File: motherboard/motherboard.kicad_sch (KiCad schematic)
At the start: 37 parts, among them J1 Conn_01x20_Pin, J3 Conn_01x20_Pin, J4 USB2.0_16P, U1 74LS573, U3 74HC132, U4 74HC245, U5 74HC245, U6 HM62256BLP, U7 R6507, U8 NE555P, U9 74HC132

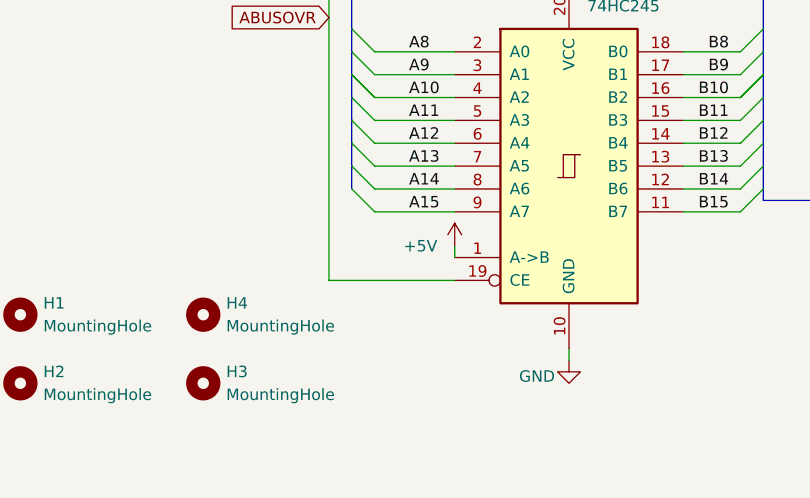
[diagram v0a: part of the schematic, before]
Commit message: Motherboard finished
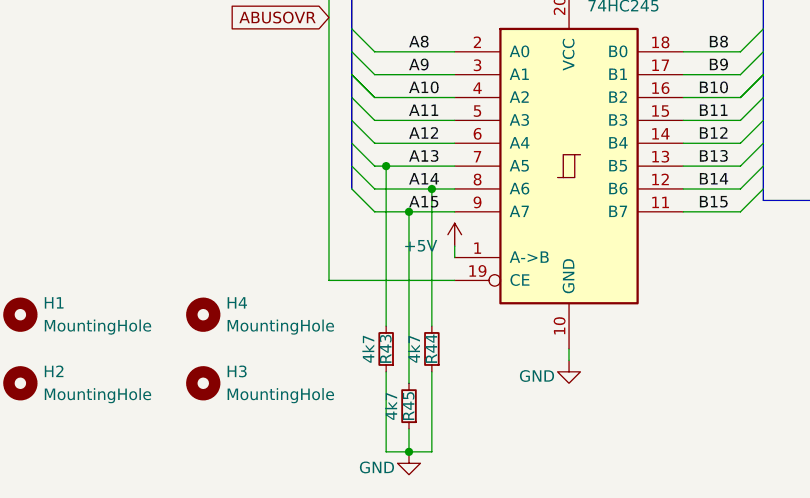
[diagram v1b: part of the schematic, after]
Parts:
- added R43, R44, R45: 4k7, Resistor_THT:R_Axial_DIN0204_L3.6mm_D1.6mm_P5.08mm_Horizontal, symbol Device:R_Small
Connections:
- net A13: now also R43.2
- net A14: now also R44.2
- net A15: now also R45.2
- net GND: now also R43.1, R44.1, R45.1
